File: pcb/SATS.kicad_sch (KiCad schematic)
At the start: 18 parts, among them J1 Raspberry_Pi_2_3, J2 A00-432-262-450, J3 AudioJack4_SwitchTR1, J4 5V, J5 3.3V, J6 Card LED, SW1 Main Door Switch, SW2 Serv Door Switch, SW3 Third Reed Switch, U1 MCP23017_SP, U2 MCP23017_SP, U3 CD40109BE, U4 IRLZ14PBF

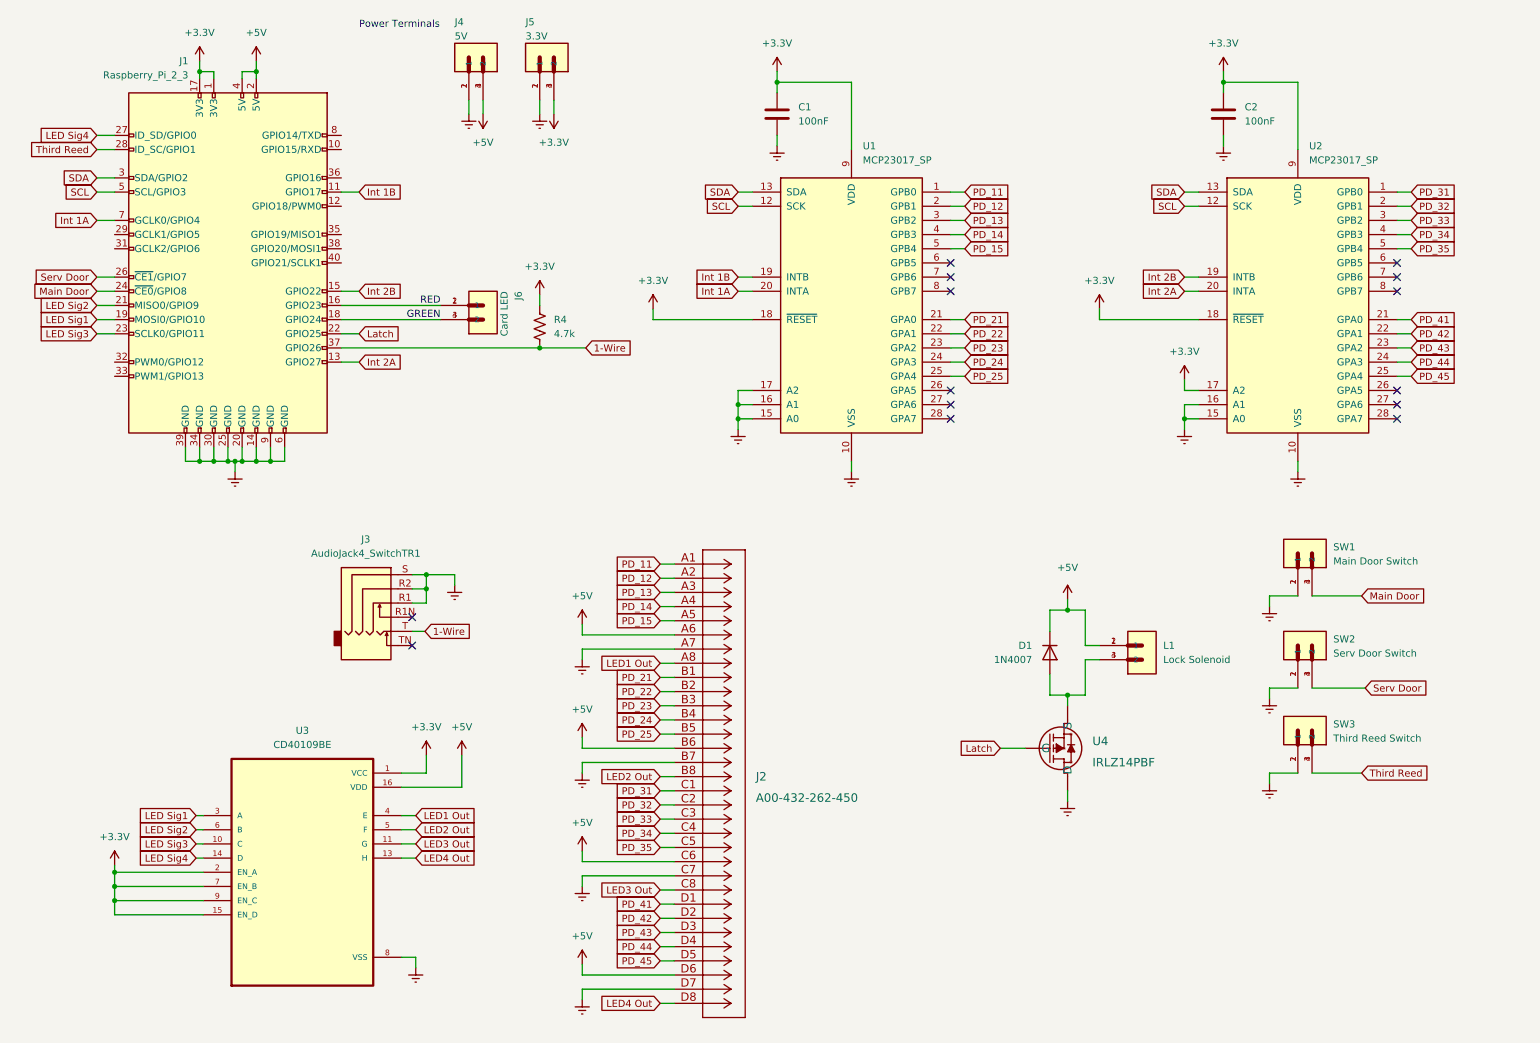
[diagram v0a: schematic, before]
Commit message: Finish Schematic
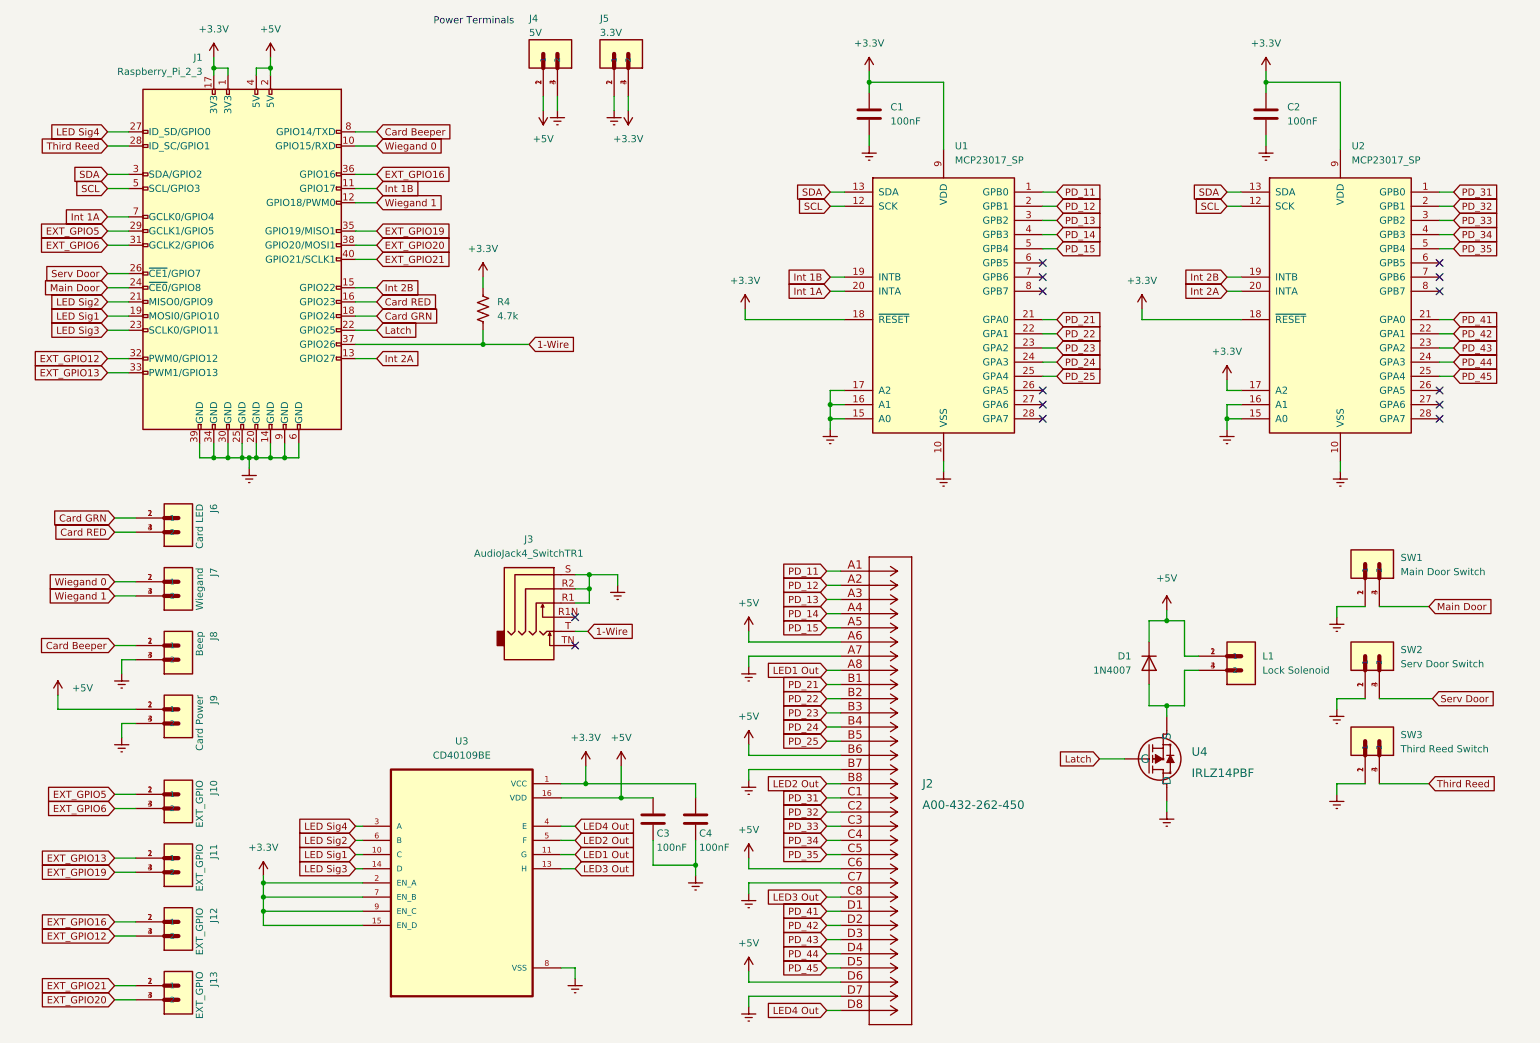
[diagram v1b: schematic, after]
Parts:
- added C3, C4: 100nF, Capacitor_THT:C_Rect_L7.0mm_W3.5mm_P5.00mm, symbol Device:C
- added J10, J11, J12, J13: EXT_GPIO, TerminalConn:PHOENIX_1862042, symbol TerminalConn:1862042
- added J7: Wiegand, TerminalConn:PHOENIX_1862042, symbol TerminalConn:1862042
- added J8: Beep, TerminalConn:PHOENIX_1862042, symbol TerminalConn:1862042
- added J9: Card Power, TerminalConn:PHOENIX_1862042, symbol TerminalConn:1862042
- J4, J5, J6: footprint PHOENIX_1862042 -> TerminalConn:PHOENIX_1862042
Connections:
- net +3V3: now also C4.1
- net +5V: now also J4.1, J4.2 (1), C3.1, J9.1, J9.2 (1); no longer J4.3 (2), J4.4 (2)
- net Earth: now also J4.3 (2), J4.4 (2), C3.2, C4.2, J8.3 (2), J8.4 (2), J9.3 (2), J9.4 (2); no longer J4.1, J4.2 (1)
- net LED Sig1: now also U3.10 (C); no longer U3.3 (A)
- net LED Sig3: now also U3.14 (D); no longer U3.10 (C)
- net LED Sig4: now also U3.3 (A); no longer U3.14 (D)
- net LED1 Out: now also U3.11 (G); no longer U3.4 (E)
- net LED3 Out: now also U3.13 (H); no longer U3.11 (G)
- net LED4 Out: now also U3.4 (E); no longer U3.13 (H)
- net Wiegand 0: now reaches J1.10 (GPIO15/RXD)
- net Wiegand 0: now also J7.1, J7.2 (1)
- net Wiegand 1: now reaches J1.12 (GPIO18/PWM0)
- net Wiegand 1: now also J7.3 (2), J7.4 (2)
- net EXT_GPIO5: now reaches J1.29 (GCLK1/GPIO5)
- net EXT_GPIO5: now also J10.1, J10.2 (1)
- net EXT_GPIO6: now reaches J1.31 (GCLK2/GPIO6)
- net EXT_GPIO6: now also J10.3 (2), J10.4 (2)
- net EXT_GPIO12: now reaches J1.32 (PWM0/GPIO12)
- net EXT_GPIO12: now also J12.3 (2), J12.4 (2)
- net EXT_GPIO13: now reaches J1.33 (PWM1/GPIO13)
- net EXT_GPIO13: now also J11.1, J11.2 (1)
- net EXT_GPIO19: now reaches J1.35 (GPIO19/MISO1)
- net EXT_GPIO19: now also J11.3 (2), J11.4 (2)
- net EXT_GPIO16: now reaches J1.36 (GPIO16)
- net EXT_GPIO16: now also J12.1, J12.2 (1)
- net EXT_GPIO20: now reaches J1.38 (GPIO20/MOSI1)
- net EXT_GPIO20: now also J13.3 (2), J13.4 (2)
- net EXT_GPIO21: now reaches J1.40 (GPIO21/SCLK1)
- net EXT_GPIO21: now also J13.1, J13.2 (1)
- net Card Beeper: now reaches J1.8 (GPIO14/TXD)
- net Card Beeper: now also J8.1, J8.2 (1)
- net GREEN renamed Card RED
- net Card RED: now also J1.16 (GPIO23); no longer J1.18 (GPIO24)
- net RED renamed Card GRN
- net Card GRN: now also J1.18 (GPIO24); no longer J1.16 (GPIO23)
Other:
- moved on the sheet: C1, C2, D1, J1, J2, J3, J4, J5, J6, L1, R4, SW1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

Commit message: neatify and reorganize
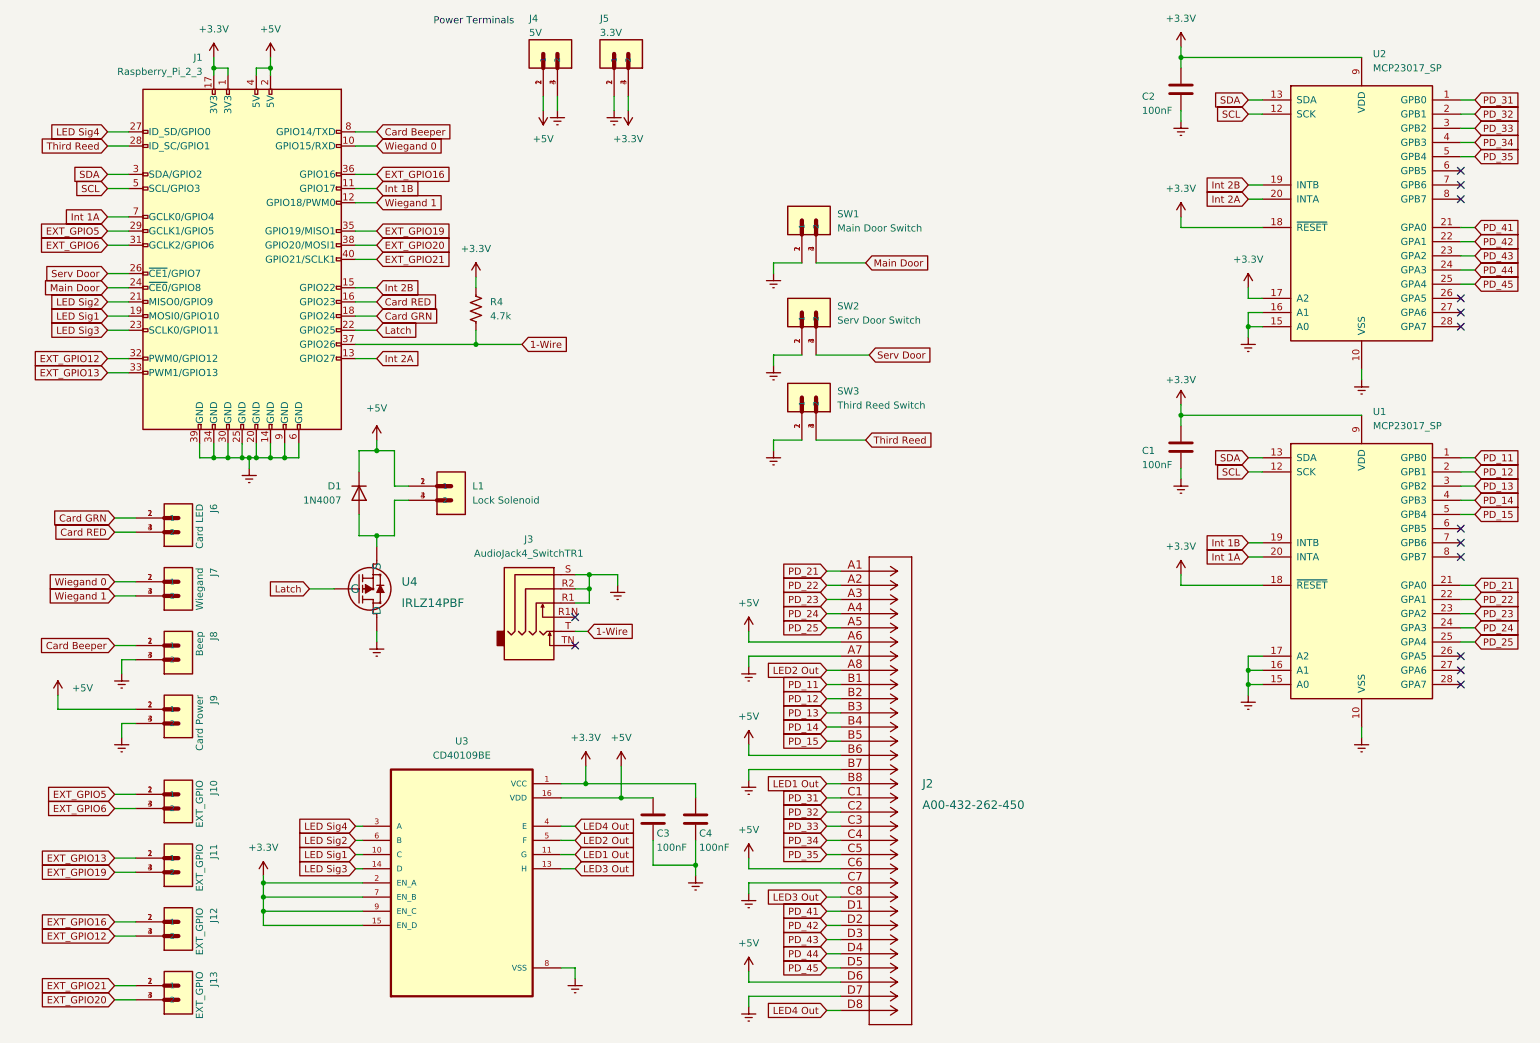
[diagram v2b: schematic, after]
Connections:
- net LED1 Out: now also J2.B8; no longer J2.A8
- net LED2 Out: now also J2.A8; no longer J2.B8
- net PD_11: now also J2.B1; no longer J2.A1
- net PD_12: now also J2.B2; no longer J2.A2
- net PD_13: now also J2.B3; no longer J2.A3
- net PD_14: now also J2.B4; no longer J2.A4
- net PD_15: now also J2.B5; no longer J2.A5
- net PD_21: now also J2.A1; no longer J2.B1
- net PD_22: now also J2.A2; no longer J2.B2
- net PD_23: now also J2.A3; no longer J2.B3
- net PD_24: now also J2.A4; no longer J2.B4
- net PD_25: now also J2.A5; no longer J2.B5
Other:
- moved on the sheet: C1, C2, D1, L1, R4, SW1, SW2, SW3, U1, U2, U4
